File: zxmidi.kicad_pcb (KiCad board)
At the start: 2 copper layers, 62.3 x 21.7 mm, 6 parts, among them J1 RJ45, J2 DIN-5_180degree, Q1 BC337

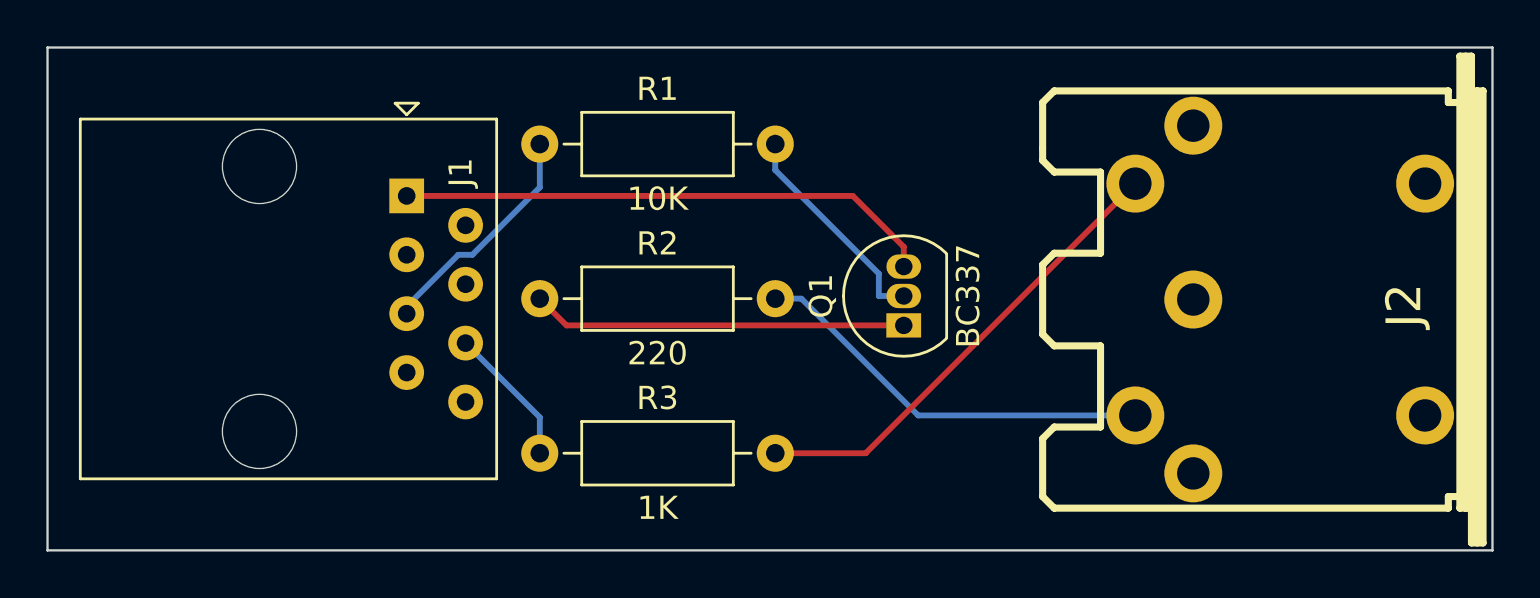
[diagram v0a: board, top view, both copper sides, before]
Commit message: Error fix
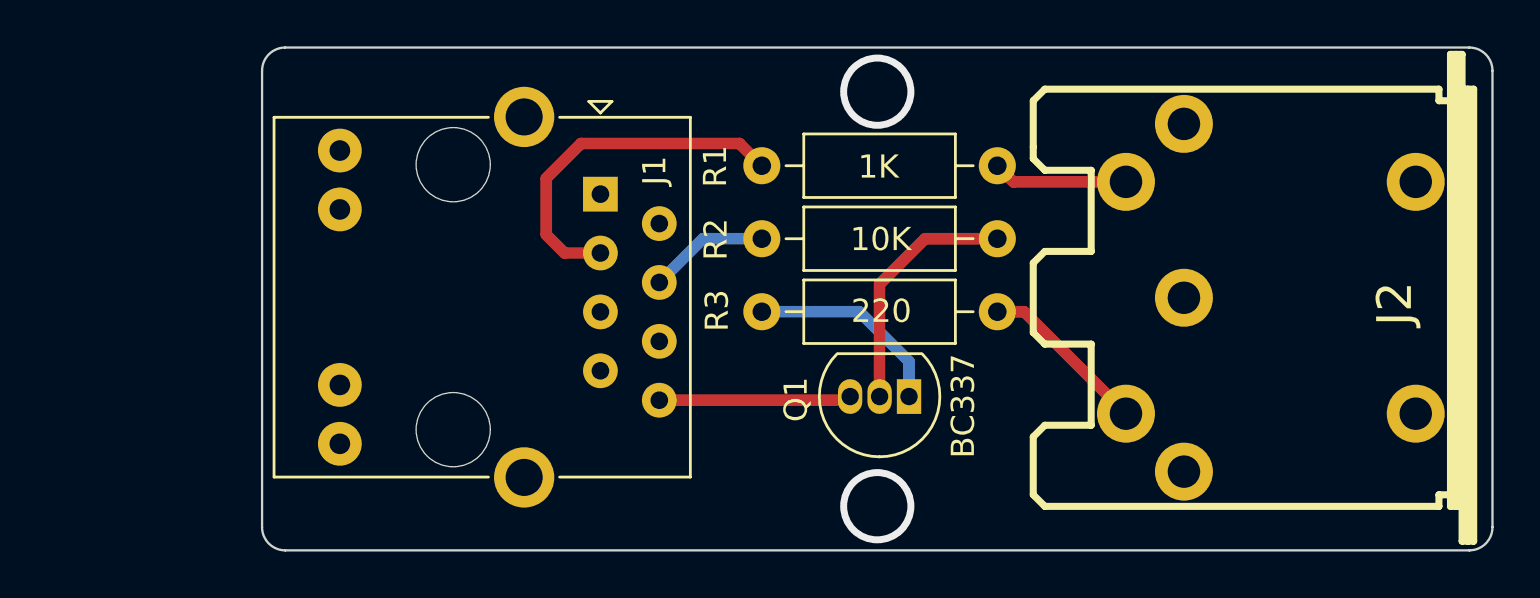
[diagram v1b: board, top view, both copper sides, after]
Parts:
- J1: footprint Connector_RJ:RJ45_Amphenol_54602-x08_Horizontal -> ZXMidi:RJ45_Amphenol_54602-x08_Horizontal
- Q1: footprint Package_TO_SOT_THT:TO-92_Inline -> ZXMidi:TO-92_Inline
- R1: renamed from R3; footprint Resistor_THT:R_Axial_DIN0207_L6.3mm_D2.5mm_P10.16mm_Horizontal -> ZXMidi:R_Axial_DIN0207_L6.3mm_D2.5mm_P10.16mm_Horizontal
- R2: renamed from R1; footprint Resistor_THT:R_Axial_DIN0207_L6.3mm_D2.5mm_P10.16mm_Horizontal -> ZXMidi:R_Axial_DIN0207_L6.3mm_D2.5mm_P10.16mm_Horizontal
- R3: renamed from R2; footprint Resistor_THT:R_Axial_DIN0207_L6.3mm_D2.5mm_P10.16mm_Horizontal -> ZXMidi:R_Axial_DIN0207_L6.3mm_D2.5mm_P10.16mm_Horizontal
- moved R1 15.7 mm to (61.4, 39.2)
- moved R2 10.4 mm to (61.4, 42.3)
- moved R3 9.60 mm to (61.4, 45.5)
- moved J1 8.36 mm to (54.4, 40.4)
- moved Q1 3.08 mm to (67.7, 49.1), turned to 180 degrees
- moved J2 0.41 mm to (82.6, 44.9)
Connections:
- J1 pad 1: Net-(Q1-E) -> unconnected-(J1-Pad1)
- J1 pad 3: unconnected-(J1-Pad3) -> Net-(J1-Pad3)
- J1 pad 4: unconnected-(J1-Pad4) -> Net-(J1-Pad4)
- J1 pad 5: Net-(J1-Pad5) -> unconnected-(J1-Pad5)
- J1 pad 6: Net-(J1-Pad6) -> unconnected-(J1-Pad6)
- J1 pad 8: unconnected-(J1-Pad8) -> Net-(Q1-E)
- R1 pad 1: Net-(J1-Pad6) -> Net-(J1-Pad3)
- R2 pad 1: Net-(J1-Pad5) -> Net-(J1-Pad4)
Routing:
- net Net-(J1-Pad3): track 0.00 -> 15.4 mm
- net Net-(Q1-E): track 23.2 -> 8.30 mm
- net Net-(J2-Pad4): track 20.3 -> 5.84 mm
- net Net-(J2-Pad5): track 17.6 -> 7.37 mm
- net Net-(J1-Pad5): track 10.0 -> 0.00 mm
- net Net-(Q1-C): track 16.2 -> 8.75 mm
- net Net-(J1-Pad6): track 6.08 -> 0.00 mm
- net Net-(J1-Pad4): track 0.00 -> 5.20 mm
- net Net-(Q1-B): track 9.48 -> 10.7 mm
- net (no net): vias 0 -> 2
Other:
- board size 62.3 x 21.7 mm -> 53.1 x 21.7 mm
